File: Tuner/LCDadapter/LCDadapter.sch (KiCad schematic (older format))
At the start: 35 parts, among them J1 Conn_02x05_Odd_Even, J2 Conn_01x01, J3 Conn_01x01, J4 Conn_01x01, J5 Conn_01x01, Q1 2N3904, SW1 SW_Push, SW2 SW_Push, SW3 SW_Push, SW4 SW_Push, SW5 SW_Push, SW6 SW_Push, U1 PCF8574, U2 LCD-016N002L

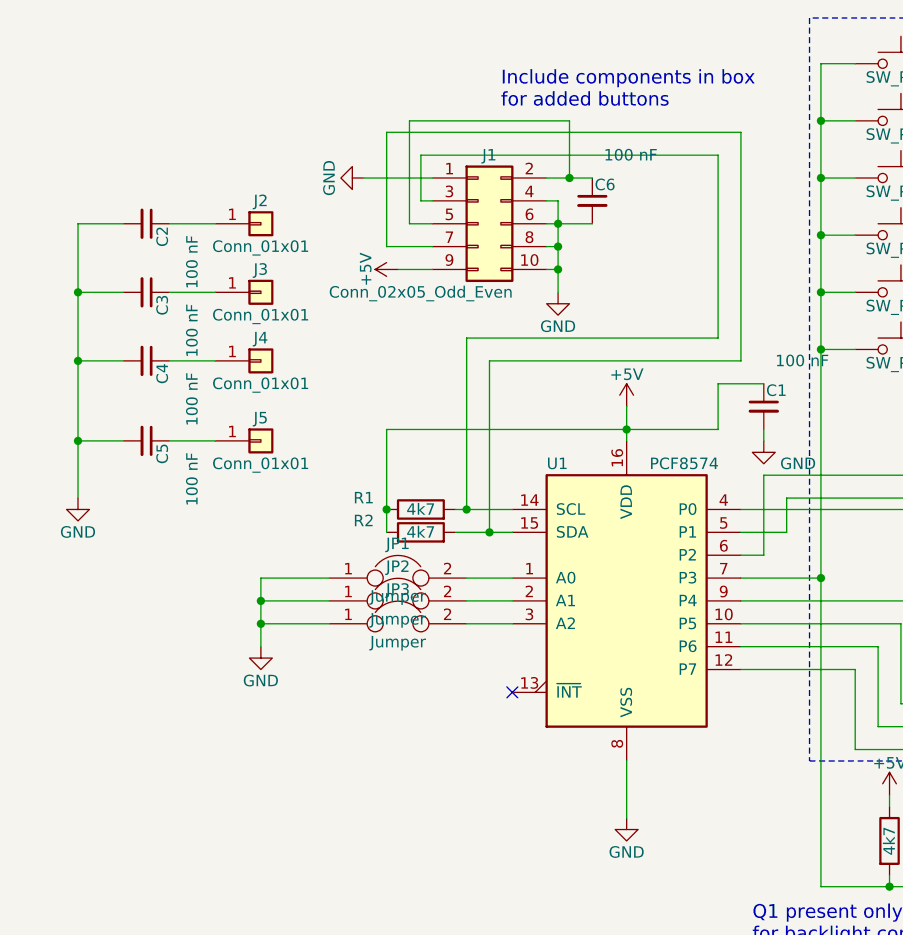
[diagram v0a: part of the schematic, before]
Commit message: LCDAdapter added dual polarity set I2C address
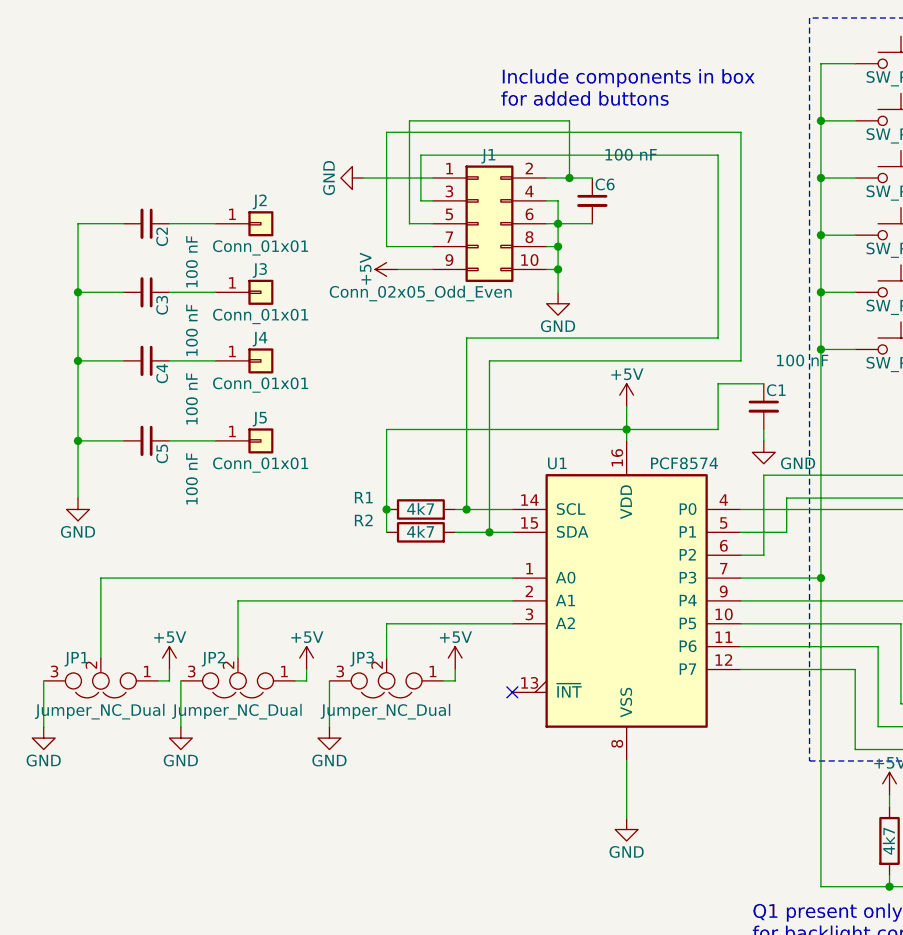
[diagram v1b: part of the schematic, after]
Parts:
- removed JP1, JP2, JP3: Jumper, Pin_Headers:Pin_Header_Straight_1x02_Pitch2.54mm, symbol Jumper
- added JP1, JP2, JP3: Jumper_NC_Dual, Pin_Headers:Pin_Header_Straight_1x03_Pitch2.54mm, symbol Jumper_NC_Dual
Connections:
- net +5V: now also JP1.1, JP2.1, JP3.1
- net GND: now also JP1.3, JP2.3, JP3.3
- net at U1.1 (A0): now also JP1.2
- net at U1.2 (A1): now also JP2.2
- net at U1.3 (A2): now also JP3.2
